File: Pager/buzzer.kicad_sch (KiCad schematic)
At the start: 1 part, among them Q1 AO3400A

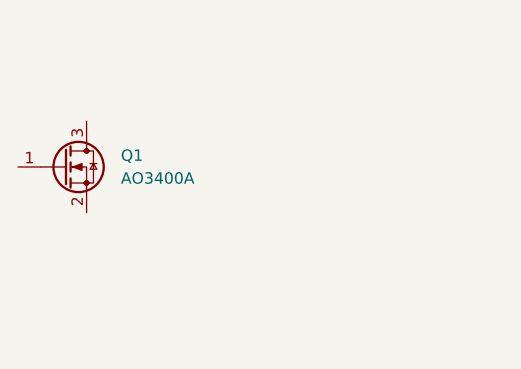
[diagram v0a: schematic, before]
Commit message: br
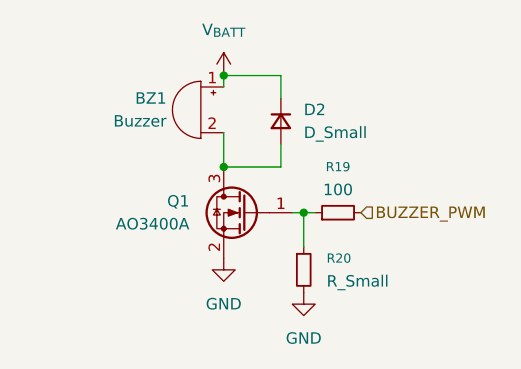
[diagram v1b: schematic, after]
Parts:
- added BZ1: Buzzer, Package_DFN_QFN:Texas_RVA_VQFN-16-1EP_3.5x3.5mm_P0.5mm_EP2.14x2.14mm_ThermalVias, symbol Device:Buzzer
- added D2: D_Small, symbol Device:D_Small
- added R19: 100, Resistor_THT:R_Array_SIP4, symbol Device:R_Small
- added R20: R_Small, Resistor_THT:R_Array_SIP4, symbol Device:R_Small
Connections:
- net at Q1.1 (G): now also R19.1, R20.1
- net GND: now reaches Q1.2 (S)
- net GND: now also R20.2
- net at Q1.3 (D): now also BZ1.2 (-), D2.2 (A)
- new net BUZZER_PWM: R19.2
- new net V_{BATT}: BZ1.1 (+), D2.1 (K)
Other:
- moved on the sheet: Q1
